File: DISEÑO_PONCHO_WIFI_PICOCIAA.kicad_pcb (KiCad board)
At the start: 2 copper layers, 51 x 30.5 mm, 15 parts, among them P1 MOUNT_HOLE, P2 MOUNT_HOLE, U1 ESP-12E

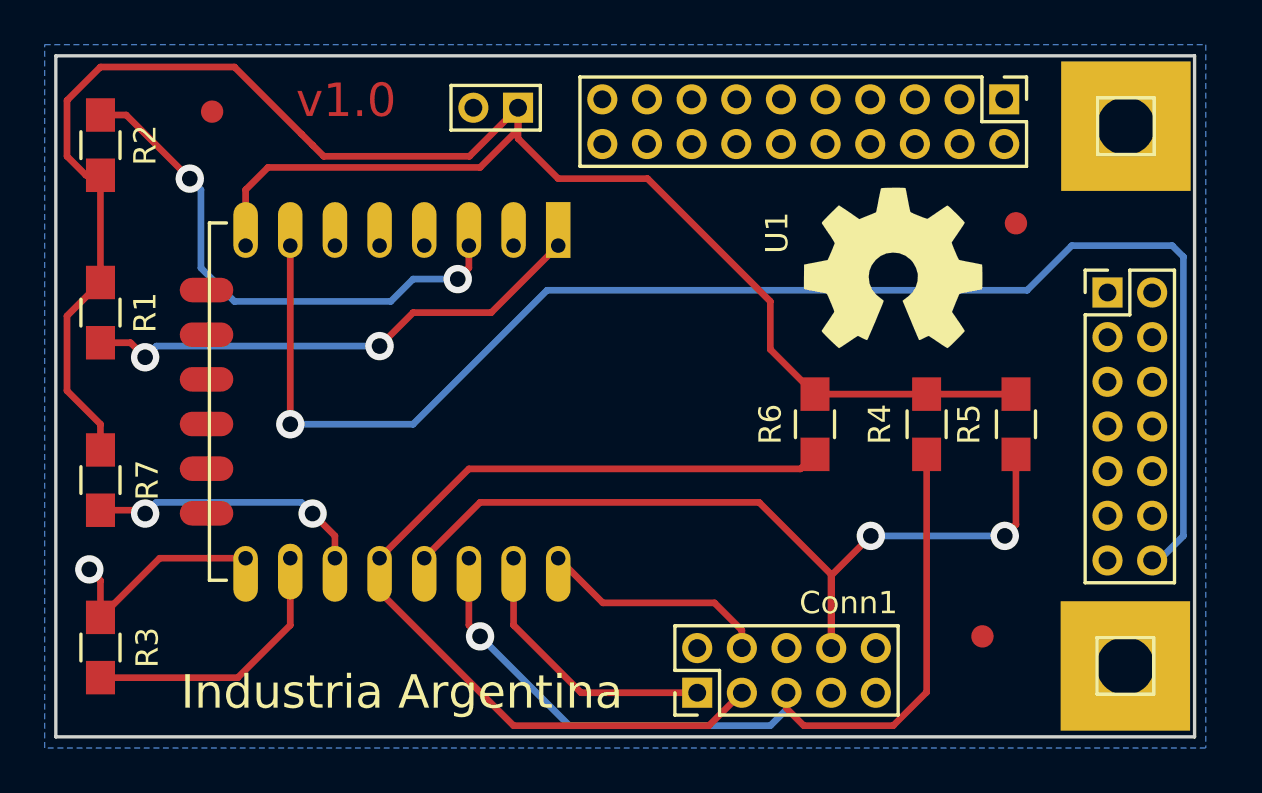
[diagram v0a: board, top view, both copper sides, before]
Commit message: Se introducen comentarios de SL
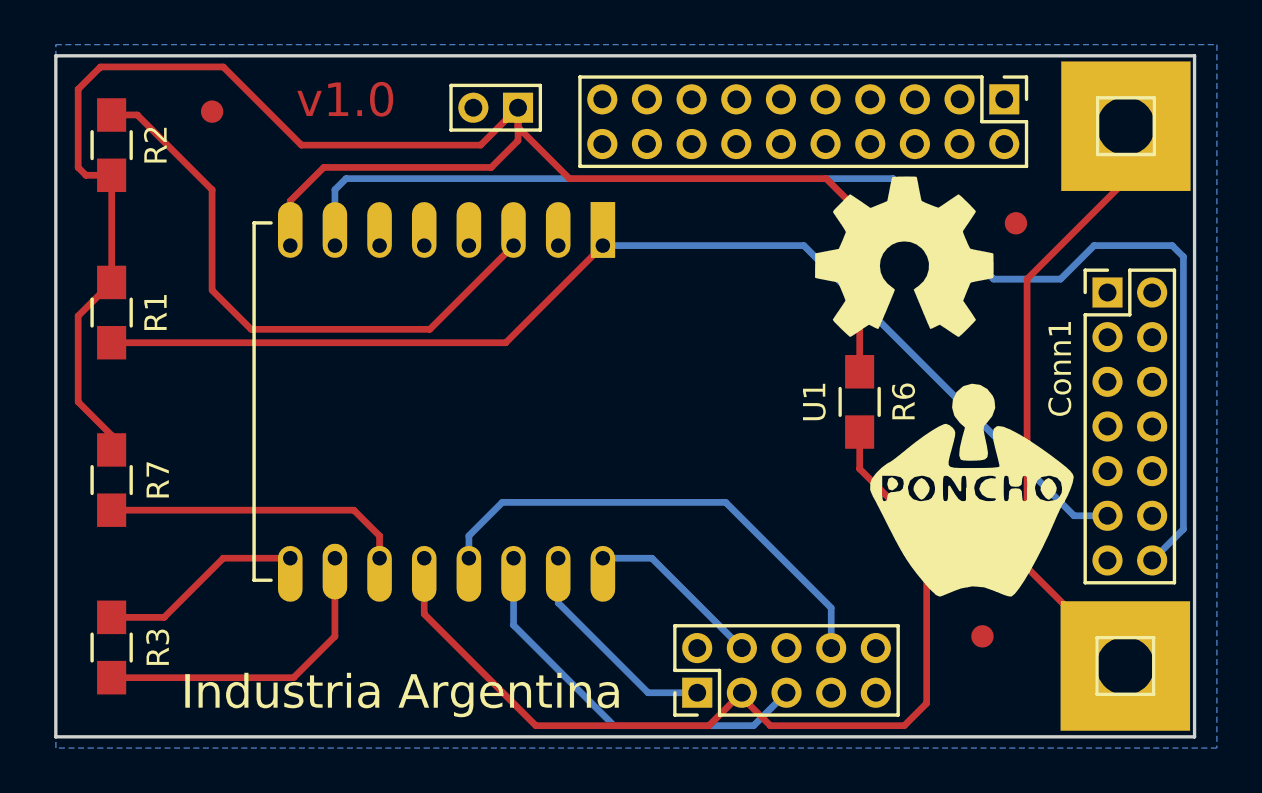
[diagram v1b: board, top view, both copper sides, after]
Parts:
- removed R4, R5: R, Resistors_SMD:R_0805_HandSoldering
- added G***: LOGO, Poncho_wifi:Logo_Poncho, F.Cu at (160.5, 103.5)
- U1: footprint pico_ciaa_ponchos:ESP-12E -> ESP-12E
- moved R6 2.24 mm to (155.5, 99.5)
- moved U1 2.00 mm to (144.0, 92.5)
- moved G101 0.71 mm to (157.5, 93.0)
- moved R1 0.50 mm to (122.0, 95.5)
- moved R2 0.50 mm to (122.0, 88.0)
- moved R3 0.50 mm to (122.0, 110.5)
- moved R7 0.50 mm to (122.0, 103.0)
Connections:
- net +3.3V renamed +3V3
- R1 pad 1: Net-(R1-Pad1) -> Net-(Conn1-Pad11)
- U1 pad 1: Net-(R1-Pad1) -> Net-(Conn1-Pad11)
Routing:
- net Net-(Conn1-Pad11): track 0.00 -> 51.4 mm
- net GND: track 9.95 -> 36.9 mm, vias 1 -> 0
- net Net-(R1-Pad1): track 22.8 -> 0.00 mm, vias 2 -> 0
- net Net-(Conn1-Pad41): track 38.7 -> 17.7 mm, vias 1 -> 0
- net Net-(Conn1-Pad44): track 39.5 -> 21.6 mm, vias 2 -> 0
- net Net-(Conn1-Pad14): track 65.9 -> 57.6 mm, vias 1 -> 0
- net +3V3: track 87.7 -> 80.6 mm
- net Net-(Conn1-Pad37): track 12.5 -> 9.89 mm
- net Net-(R2-Pad1): track 23.6 -> 26.2 mm, vias 2 -> 0
- net Net-(Conn1-Pad40): track 10.4 -> 7.89 mm
- net Net-(R3-Pad2): track 12.5 -> 14.3 mm
- net Net-(R7-Pad2): track 12.4 -> 13.5 mm, vias 2 -> 0
